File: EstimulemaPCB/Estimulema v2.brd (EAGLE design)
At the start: 151 x 162 mm, 158 parts, among them IC3 74AC14N, IC4 ISO7240S, J1 JUMPERS12MM, J2 J15MM, J3 J_7MM, J4 JUMPERS5MM, J5 JUMPERS7MM, J6 J7MM, K2 HC-06, Q17 TIP48, Q18 TIP50, Q19 TIP50_TH, Q20 TIP50, Q21 TIP50_TH, Q22 TIP48, Q23 TIP48_TH, Q24 TIP48_TH, Q33 TIP48, Q34 TIP50, Q35 TIP50_TH, Q36 TIP50, Q37 TIP50_TH, Q38 TIP48, Q39 TIP48_TH, Q40 TIP48_TH, X1HV+ CONECTOR_5.08, X2+15- CONECTOR_5.08, X3HV- CONECTOR_5.08

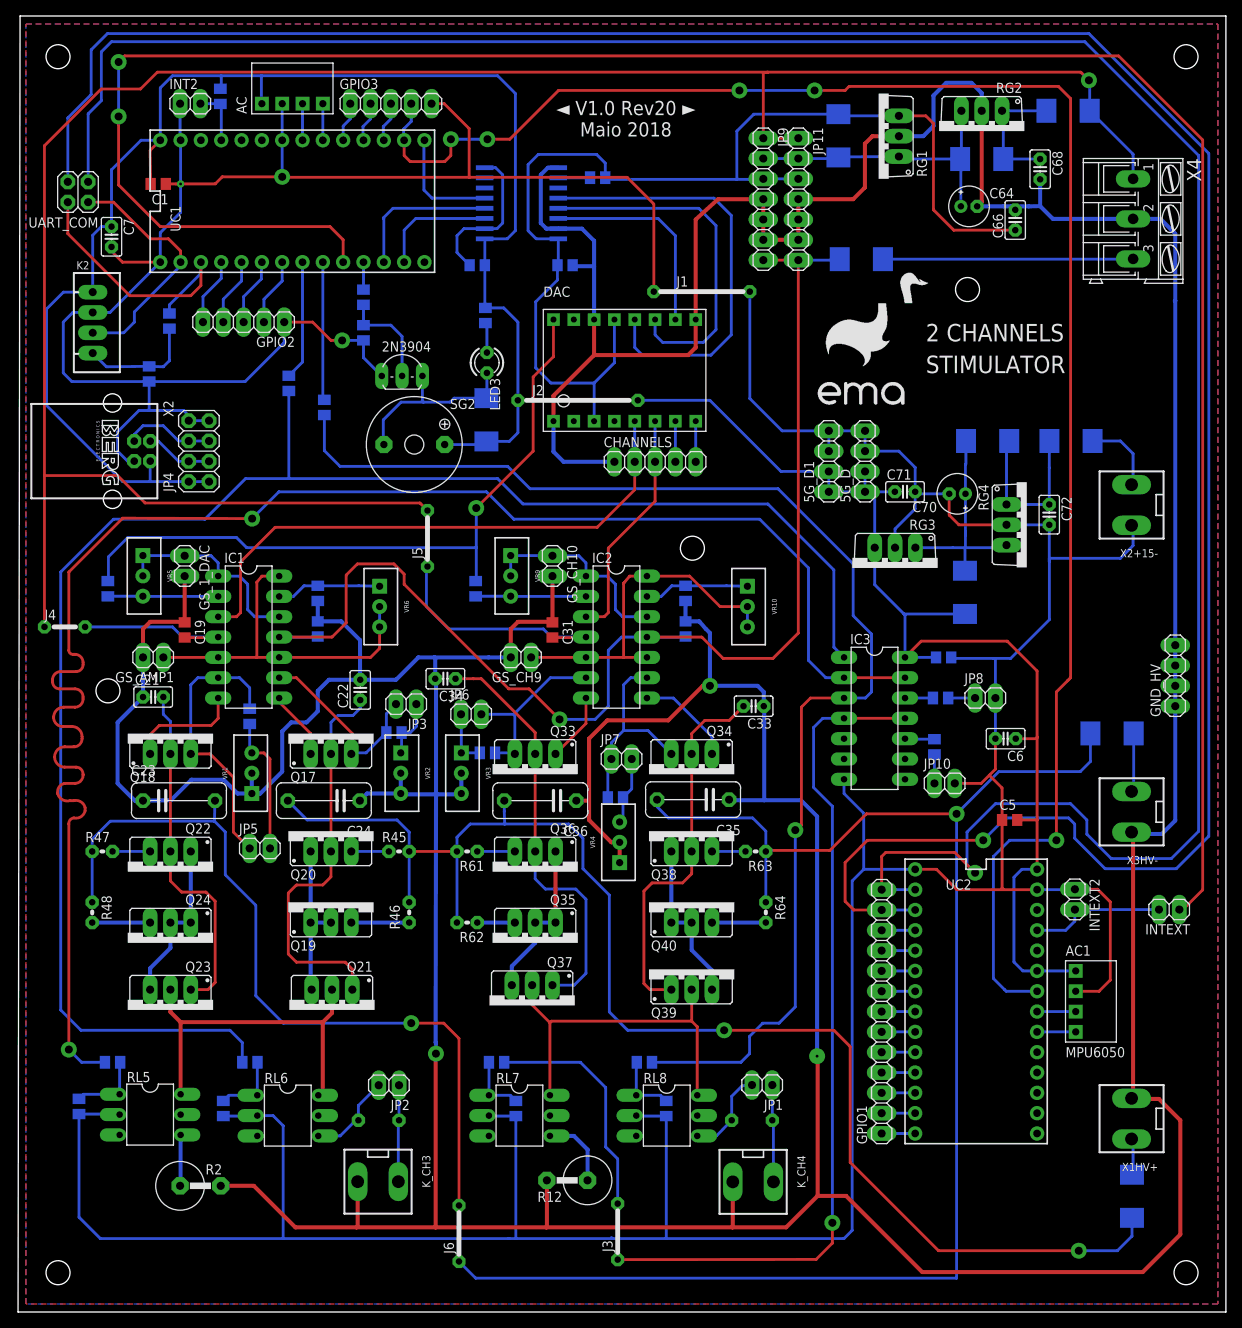
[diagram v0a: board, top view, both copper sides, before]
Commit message: Actualizacion de PCB
Version corregida con todo
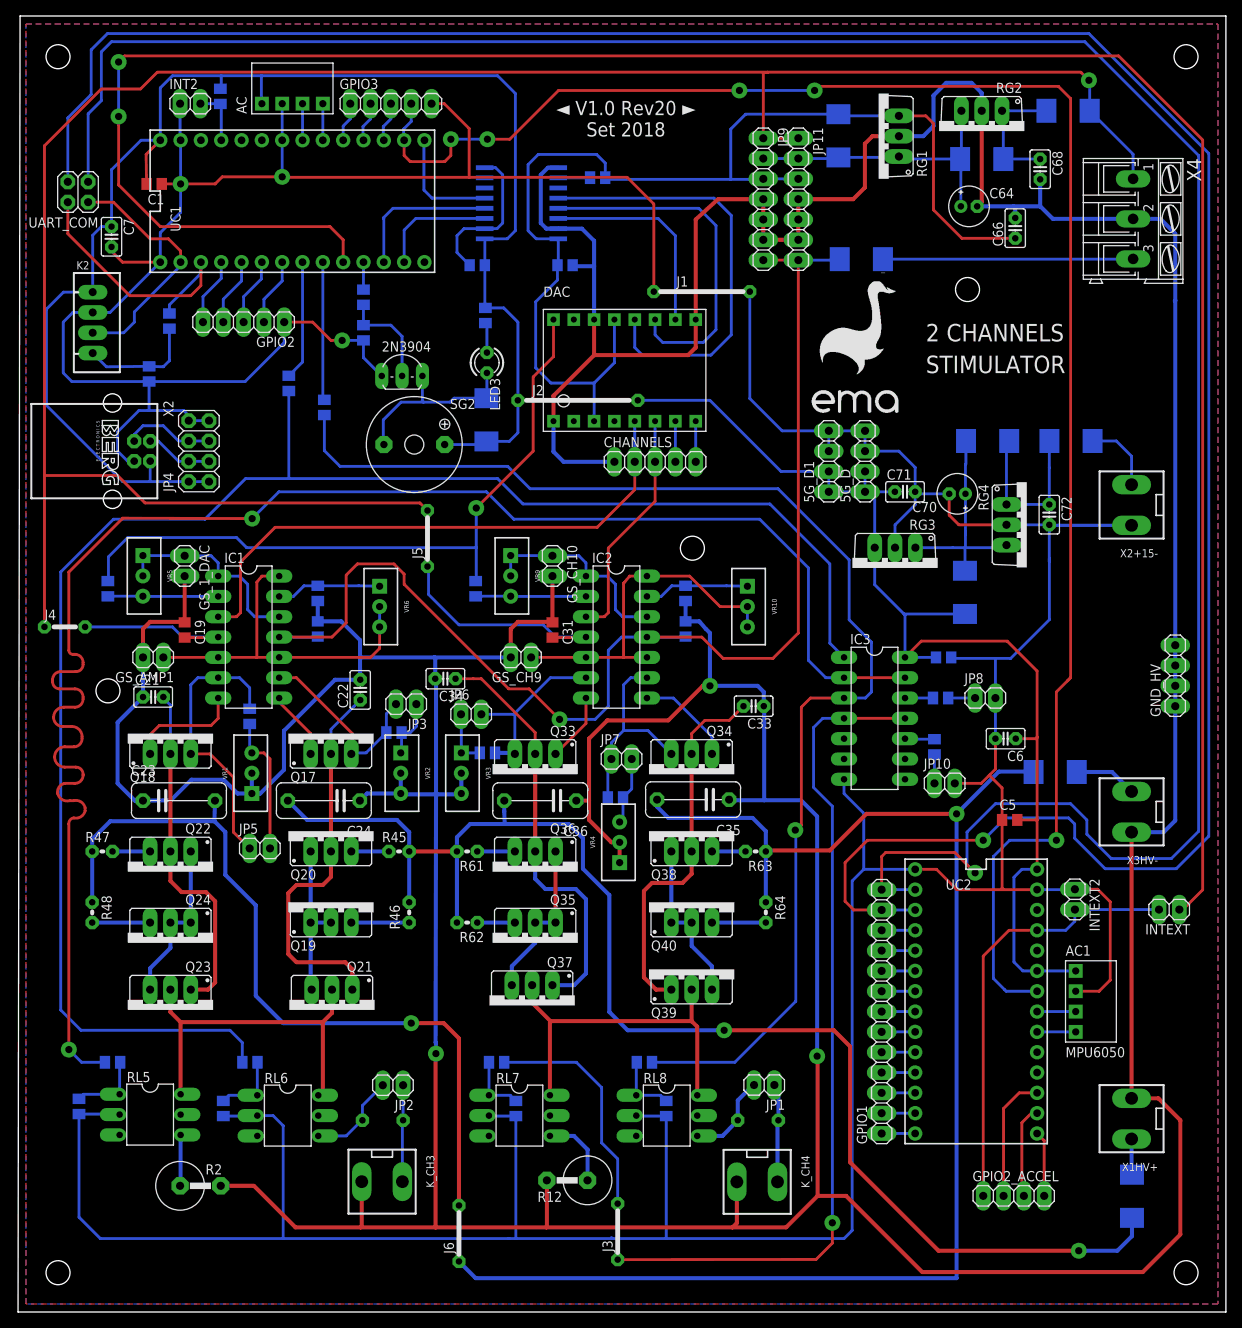
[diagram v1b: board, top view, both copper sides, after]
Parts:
- added GPIO2_ACCEL: (no value), pinhead:1X04
- moved D1 8.59 mm to (130.7, 117.5)
- moved C66 1.02 mm to (125.7, 185.5)
- moved R1 0.76 mm to (93.5, 74.0)
- moved K_CH4 0.51 mm to (93.4, 66.3)
- moved C1 0.51 mm to (18.0, 191.0)
- moved K_CH3 0.51 mm to (46.5, 66.3)
- moved R5 0.51 mm to (46.6, 74.0)
- moved JP2 0.51 mm to (47.9, 78.3)
- moved JP1 0.25 mm to (94.3, 78.4)
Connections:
- new net N$37: GPIO2_ACCEL.4, UC2.13
- new net N$39: GPIO2_ACCEL.3, UC2.14/A0
- new net N$40: GPIO2_ACCEL.2, UC2.15/A1
- net N$1: now also GPIO2_ACCEL.1
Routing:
- net N$1: track 17.4 -> 55.4 mm
- net N$40: track 0.00 -> 15.9 mm
- net N$39: track 0.00 -> 11.6 mm
- net HV-: track 294.1 -> 283.0 mm
- net N$37: track 0.00 -> 8.17 mm
- net GND_D: track 645.6 -> 642.5 mm
- net C_CH2: track 162.8 -> 161.2 mm
- net +5_HV: track 143.2 -> 144.5 mm
- net GND_HV: track 815.3 -> 814.0 mm, vias 4 -> 3
- net +15_HV: track 324.6 -> 323.4 mm
- net N$112: track 49.8 -> 48.7 mm
- net 1HV-: track 7.60 -> 8.23 mm
- net N$8: track 11.3 -> 11.8 mm
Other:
- board text added: "◄ V1.0 Rev20 ► Set 2018"
- board text removed: "◄ V1.0 Rev20 ► Maio 2018"
